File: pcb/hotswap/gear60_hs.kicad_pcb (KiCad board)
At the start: 2 copper layers, 284.2 x 93.7 mm, 185 parts, among them J1 USB_C_Receptacle_USB2.0, J3 Conn_01x05, U1 XC6206PxxxMR, U2 SRV05-4, U3 W25Q128JVS, U4 RP2040, Y1 Crystal_GND24

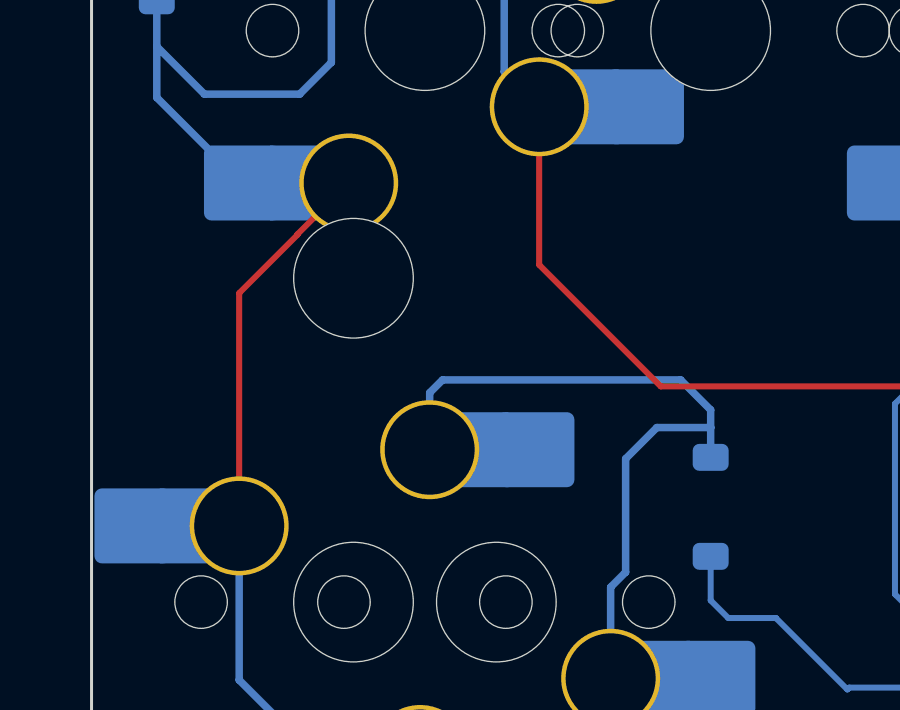
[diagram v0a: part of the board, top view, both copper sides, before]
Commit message: Add files via upload
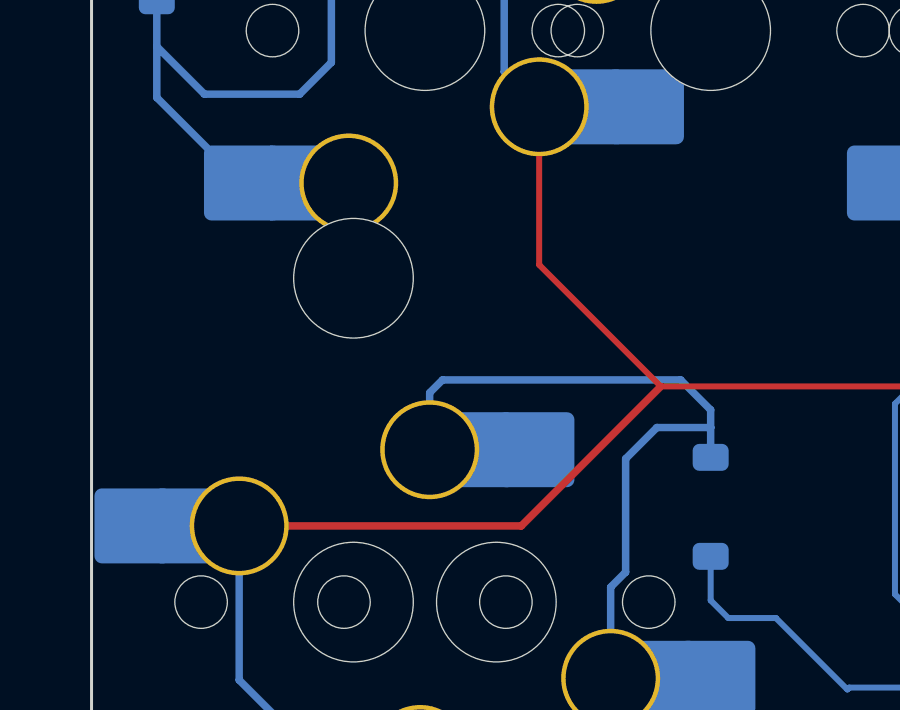
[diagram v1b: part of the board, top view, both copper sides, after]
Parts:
- F1: value MF-MSMF050-2 500mA -> MF-MSMF050-2
- J1: value USB_C_Receptacle_USB2.0 -> TYPE-C-31-M-12
- U1: value XC6206PxxxMR -> XC6206P332MR
- U3: value W25Q128JVS -> W25Q128JVSIQ
- Y1: value Crystal_GND24 -> X322512MSB4SI
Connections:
- MX63 pad 1: Net-(D48-A) -> COL0
- MX73 pad 2: Net-(D48-A) -> COL0
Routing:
- net COL0: track 187.9 -> 212.5 mm
- net Net-(D48-A): track 55.3 -> 33.8 mm
